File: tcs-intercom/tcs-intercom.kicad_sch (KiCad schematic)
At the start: 13 parts

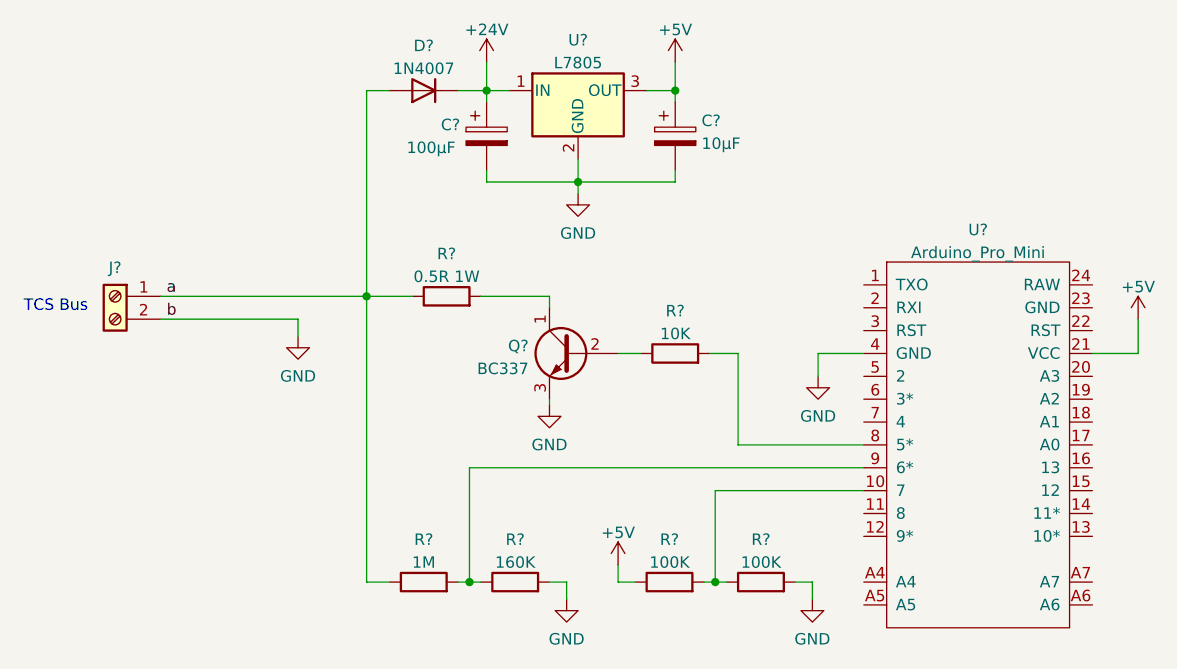
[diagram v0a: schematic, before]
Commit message: Updated tcs-intercom
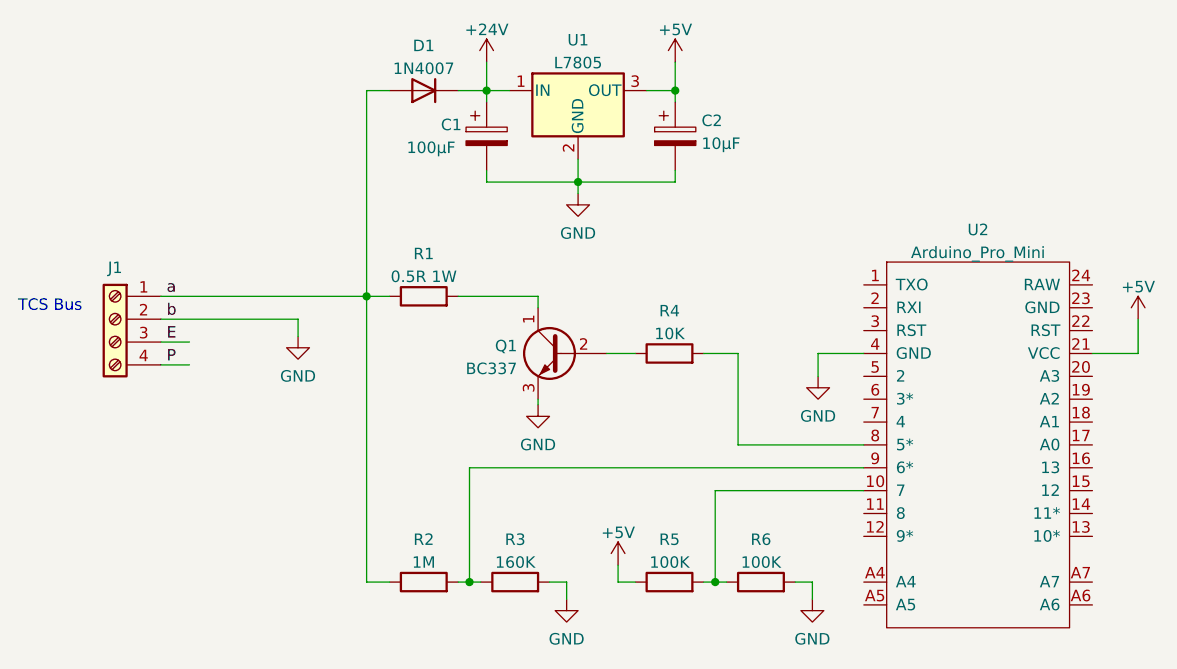
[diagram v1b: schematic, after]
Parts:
- removed J?: Screw_Terminal_01x02, symbol Connector:Screw_Terminal_01x02
- added J1: Screw_Terminal_01x04, symbol Connector:Screw_Terminal_01x04
- gave numbers to parts that had none: 12
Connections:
- net GND: now also J1.2 (Pin_2)
- net a: now also J1.1 (Pin_1)
- new net E: J1.3 (Pin_3)
- new net P: J1.4 (Pin_4)
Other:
- moved on the sheet: Q1, R1, R4

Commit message: Updated tcs-intercom
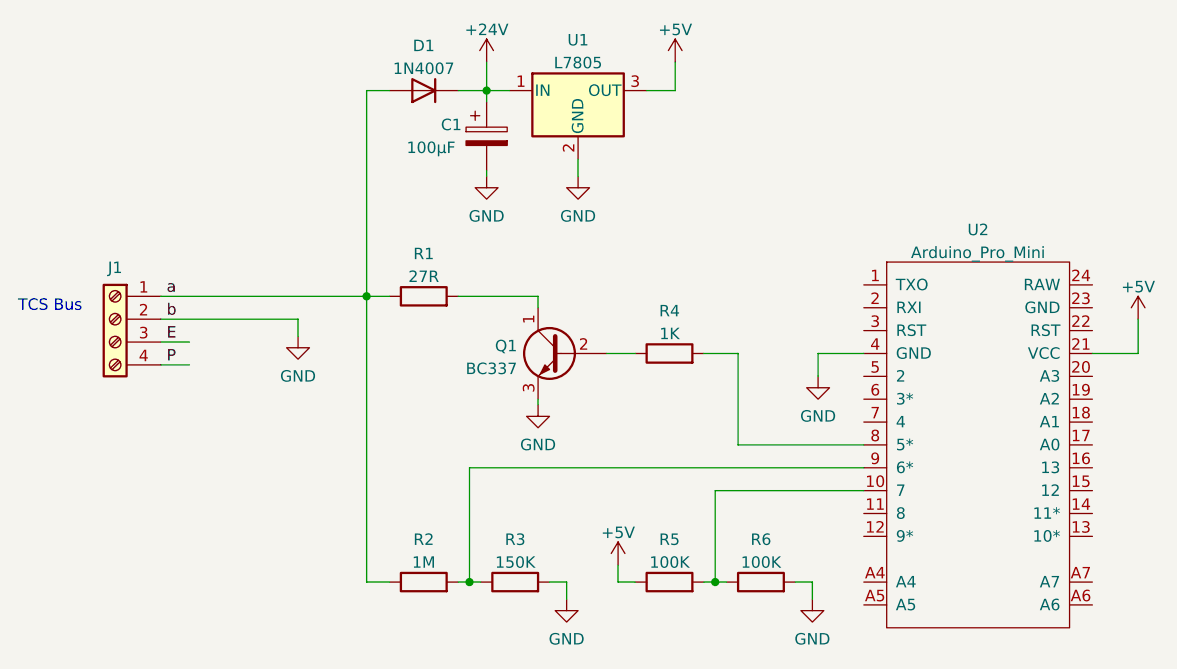
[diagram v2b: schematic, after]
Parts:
- removed C2: 10µF, symbol Device:C_Polarized
- R1: value 0.5R 1W -> 27R
- R3: value 160K -> 150K
- R4: value 10K -> 1K
